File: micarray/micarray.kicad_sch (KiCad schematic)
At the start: 37 parts, among them IC1 74LCX125MTCX, J1 Previous, J2 Next, J3 MCHStreamer J3

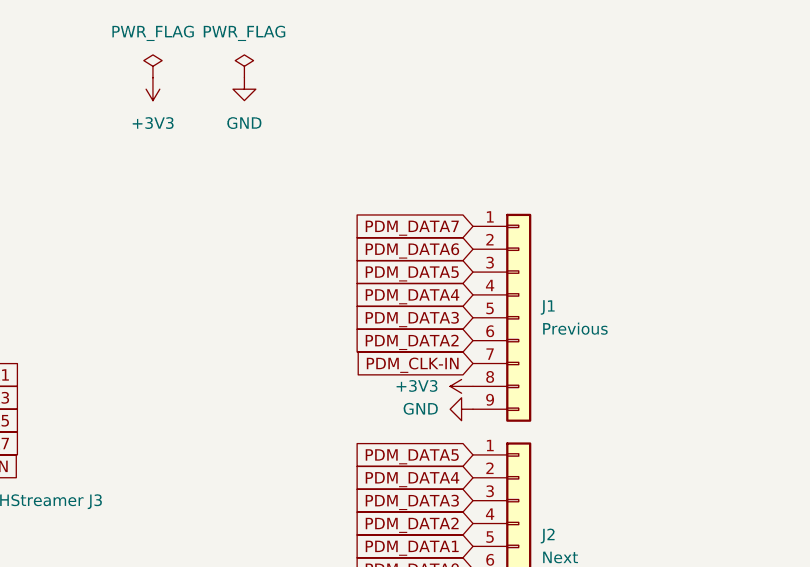
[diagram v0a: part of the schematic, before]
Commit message: save
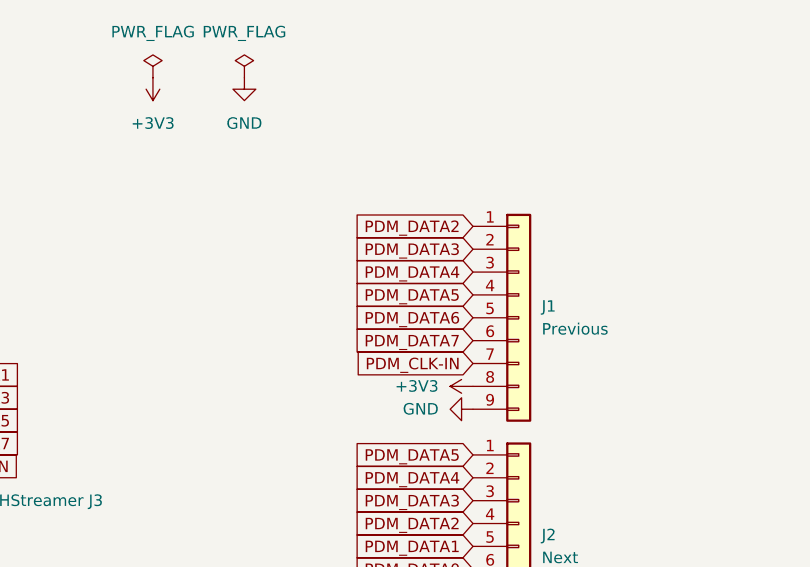
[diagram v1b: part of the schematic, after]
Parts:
- J1: footprint Connector_PinSocket_2.54mm:PinSocket_1x09_P2.54mm_Horizontal -> Connector_PinSocket_2.54mm:PinSocket_2x05_P2.54mm_Horizontal
- J2: footprint Connector_PinHeader_2.54mm:PinHeader_1x09_P2.54mm_Horizontal -> Connector_PinHeader_2.54mm:PinHeader_2x05_P2.54mm_Horizontal
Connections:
- net PDM_DATA2: now also J1.1 (Pin_1); no longer J1.6 (Pin_6)
- net PDM_DATA3: now also J1.2 (Pin_2); no longer J1.5 (Pin_5)
- net PDM_DATA4: now also J1.3 (Pin_3); no longer J1.4 (Pin_4)
- net PDM_DATA5: now also J1.4 (Pin_4); no longer J1.3 (Pin_3)
- net PDM_DATA6: now also J1.5 (Pin_5); no longer J1.2 (Pin_2)
- net PDM_DATA7: now also J1.6 (Pin_6); no longer J1.1 (Pin_1)
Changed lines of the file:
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@@
 		)
 	)
-	(global_label "PDM_DATA5"
-		(shape input)
-		(at 292.1 50.8 180)
-		(fields_autoplaced yes)
-		(effects
-			(font
-				(size 1.27 1.27)
-			)
-			(justify right)
-		)
-		(property "Intersheetrefs" "${INTERSHEET_REFS}"
-			(at 278.5315 50.8 0)
-			(effects
-				(font
-					(size 1.27 1.27)
-				)
-				(justify right)
-				(hide yes)
-			)
-		)
-	)
-	(global_label "PDM_DATA2"
-		(shape input)
-		(at 292.1 58.42 180)
-		(fields_autoplaced yes)
-		(effects
-			(font
-				(size 1.27 1.27)
-			)
-			(justify right)
-		)
-		(property "Intersheetrefs" "${INTERSHEET_REFS}"
-			(at 278.5315 58.42 0)
-			(effects
-				(font
-					(size 1.27 1.27)
-				)
-				(justify right)
-				(hide yes)
-			)
-		)
-	)
 	(global_label "PDM_CLK-IN"
 		(shape input)
@@
 		)
 	)
-	(global_label "PDM_DATA3"
+	(global_label "PDM_DATA0"
 		(shape input)
-		(at 292.1 55.88 180)
+		(at 215.9 62.23 180)
 		(fields_autoplaced yes)
 		(effects
@@
 		)
 		(property "Intersheetrefs" "${INTERSHEET_REFS}"
-			(at 278.5315 55.88 0)
+			(at 202.3315 62.23 0)
 			(effects
 				(font
@@
 		)
 	)
-	(global_label "PDM_DATA0"
+	(global_label "PDM_DATA3"
 		(shape input)
-		(at 215.9 62.23 180)
+		(at 292.1 48.26 180)
 		(fields_autoplaced yes)
 		(effects
@@
 		)
 		(property "Intersheetrefs" "${INTERSHEET_REFS}"
-			(at 202.3315 62.23 0)
+			(at 278.5315 48.26 0)
 			(effects
 				(font
@@
 		)
 	)
+	(global_label "PDM_CLK0"
+		(shape input)
+		(at 347.98 53.34 180)
+		(fields_autoplaced yes)
+		(effects
+			(font
+				(size 1.27 1.27)
+			)
+			(justify right)
+		)
+		(property "Intersheetrefs" "${INTERSHEET_REFS}"
+			(at 335.2582 53.34 0)
+			(effects
+				(font
+					(size 1.27 1.27)
+				)
+				(justify right)
+				(hide yes)
+			)
+		)
+	)
 	(global_label "PDM_DATA6"
 		(shape input)
-		(at 292.1 48.26 180)
+		(at 292.1 55.88 180)
 		(fields_autoplaced yes)
 		(effects
@@
 		)
 		(property "Intersheetrefs" "${INTERSHEET_REFS}"
-			(at 278.5315 48.26 0)
+			(at 278.5315 55.88 0)
 			(effects
 				(font
@@
 		)
 	)
-	(global_label "PDM_CLK0"
+	(global_label "PDM_DATA7"
 		(shape input)
-		(at 347.98 53.34 180)
+		(at 292.1 58.42 180)
 		(fields_autoplaced yes)
 		(effects
@@
 		)
 		(property "Intersheetrefs" "${INTERSHEET_REFS}"
-			(at 335.2582 53.34 0)
+			(at 278.5315 58.42 0)
 			(effects
 				(font
@@
 		)
 	)
+	(global_label "PDM_DATA5"
+		(shape input)
+		(at 292.1 53.34 180)
+		(fields_autoplaced yes)
+		(effects
+			(font
+				(size 1.27 1.27)
+			)
+			(justify right)
+		)
+		(property "Intersheetrefs" "${INTERSHEET_REFS}"
+			(at 278.5315 53.34 0)
+			(effects
+				(font
+					(size 1.27 1.27)
+				)
+				(justify right)
+				(hide yes)
+			)
+		)
+	)
 	(global_label "PDM_DATA4"
 		(shape input)
@@
 	(global_label "PDM_DATA4"
 		(shape input)
-		(at 292.1 53.34 180)
+		(at 292.1 50.8 180)
 		(fields_autoplaced yes)
 		(effects
@@
 		)
 		(property "Intersheetrefs" "${INTERSHEET_REFS}"
-			(at 278.5315 53.34 0)
+			(at 278.5315 50.8 0)
 			(effects
 				(font
@@
 		)
 	)
-	(global_label "PDM_DATA7"
+	(global_label "PDM_DATA2"
 		(shape input)
 		(at 292.1 45.72 180)
@@
 			)
 		)
-		(property "Footprint" "Connector_PinSocket_2.54mm:PinSocket_1x09_P2.54mm_Horizontal"
+		(property "Footprint" "Connector_PinSocket_2.54mm:PinSocket_2x05_P2.54mm_Horizontal"
 			(at 297.18 55.88 0)
 			(effects
@@
 			)
 		)
-		(property "Footprint" "Connector_PinHeader_2.54mm:PinHeader_1x09_P2.54mm_Horizontal"
+		(property "Footprint" "Connector_PinHeader_2.54mm:PinHeader_2x05_P2.54mm_Horizontal"
 			(at 297.18 81.28 0)
 			(effects
